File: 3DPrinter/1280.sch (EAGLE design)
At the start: 39 parts, among them IC1 ATMEGA1280-16AU, IC2 7805DT, IC3 CP2102, IC4 X, IC5 Y, IC6 Z, IC7 E0, IC8 E1, J1 22-27-2041-04, J2 22-27-2041-04, J3 22-27-2041-04, J4 22-27-2041-04, J5 22-27-2041-04, Q1 16 MHz, X1 PN61729-S, X2 CON-5.08-03P, X3 CON-5.08-03P, X4 CON-7.62-02P

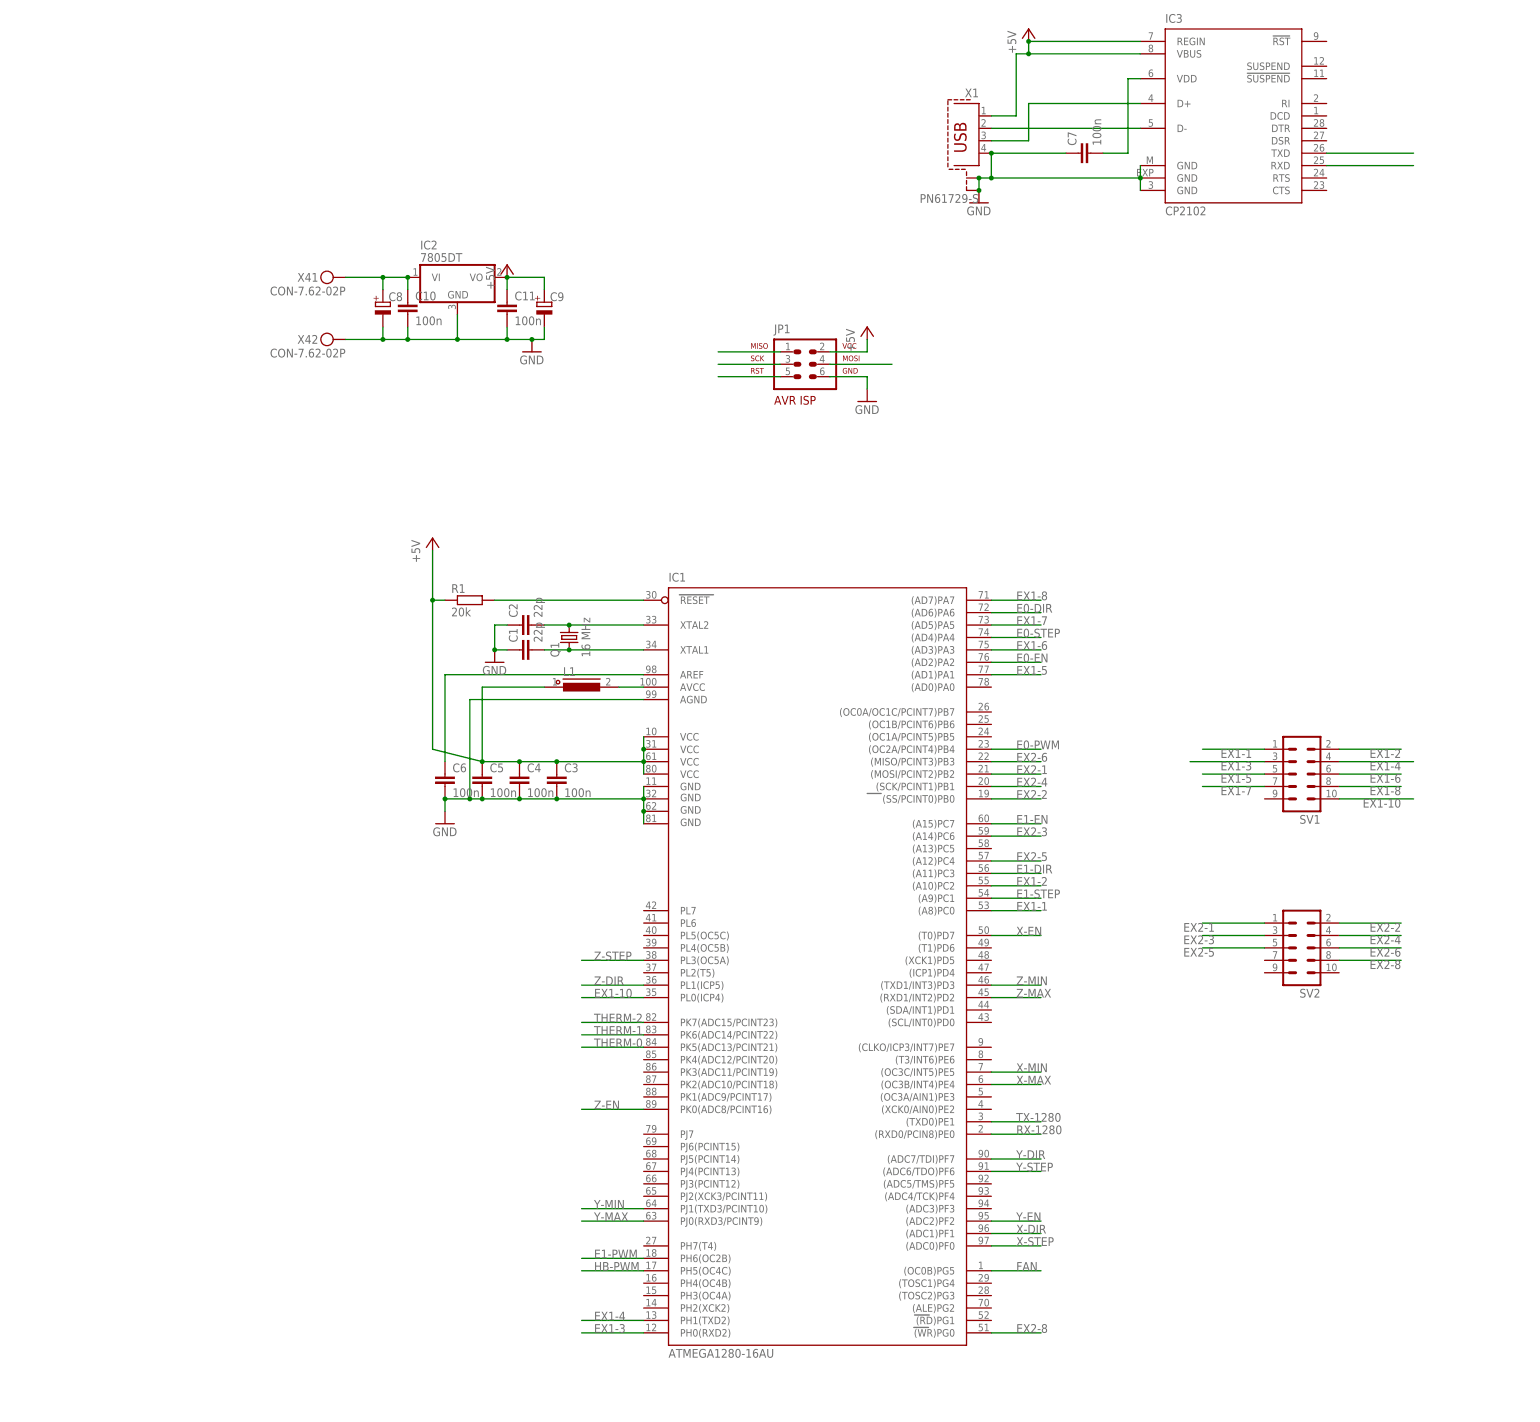
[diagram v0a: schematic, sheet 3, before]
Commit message: полная ардуйня
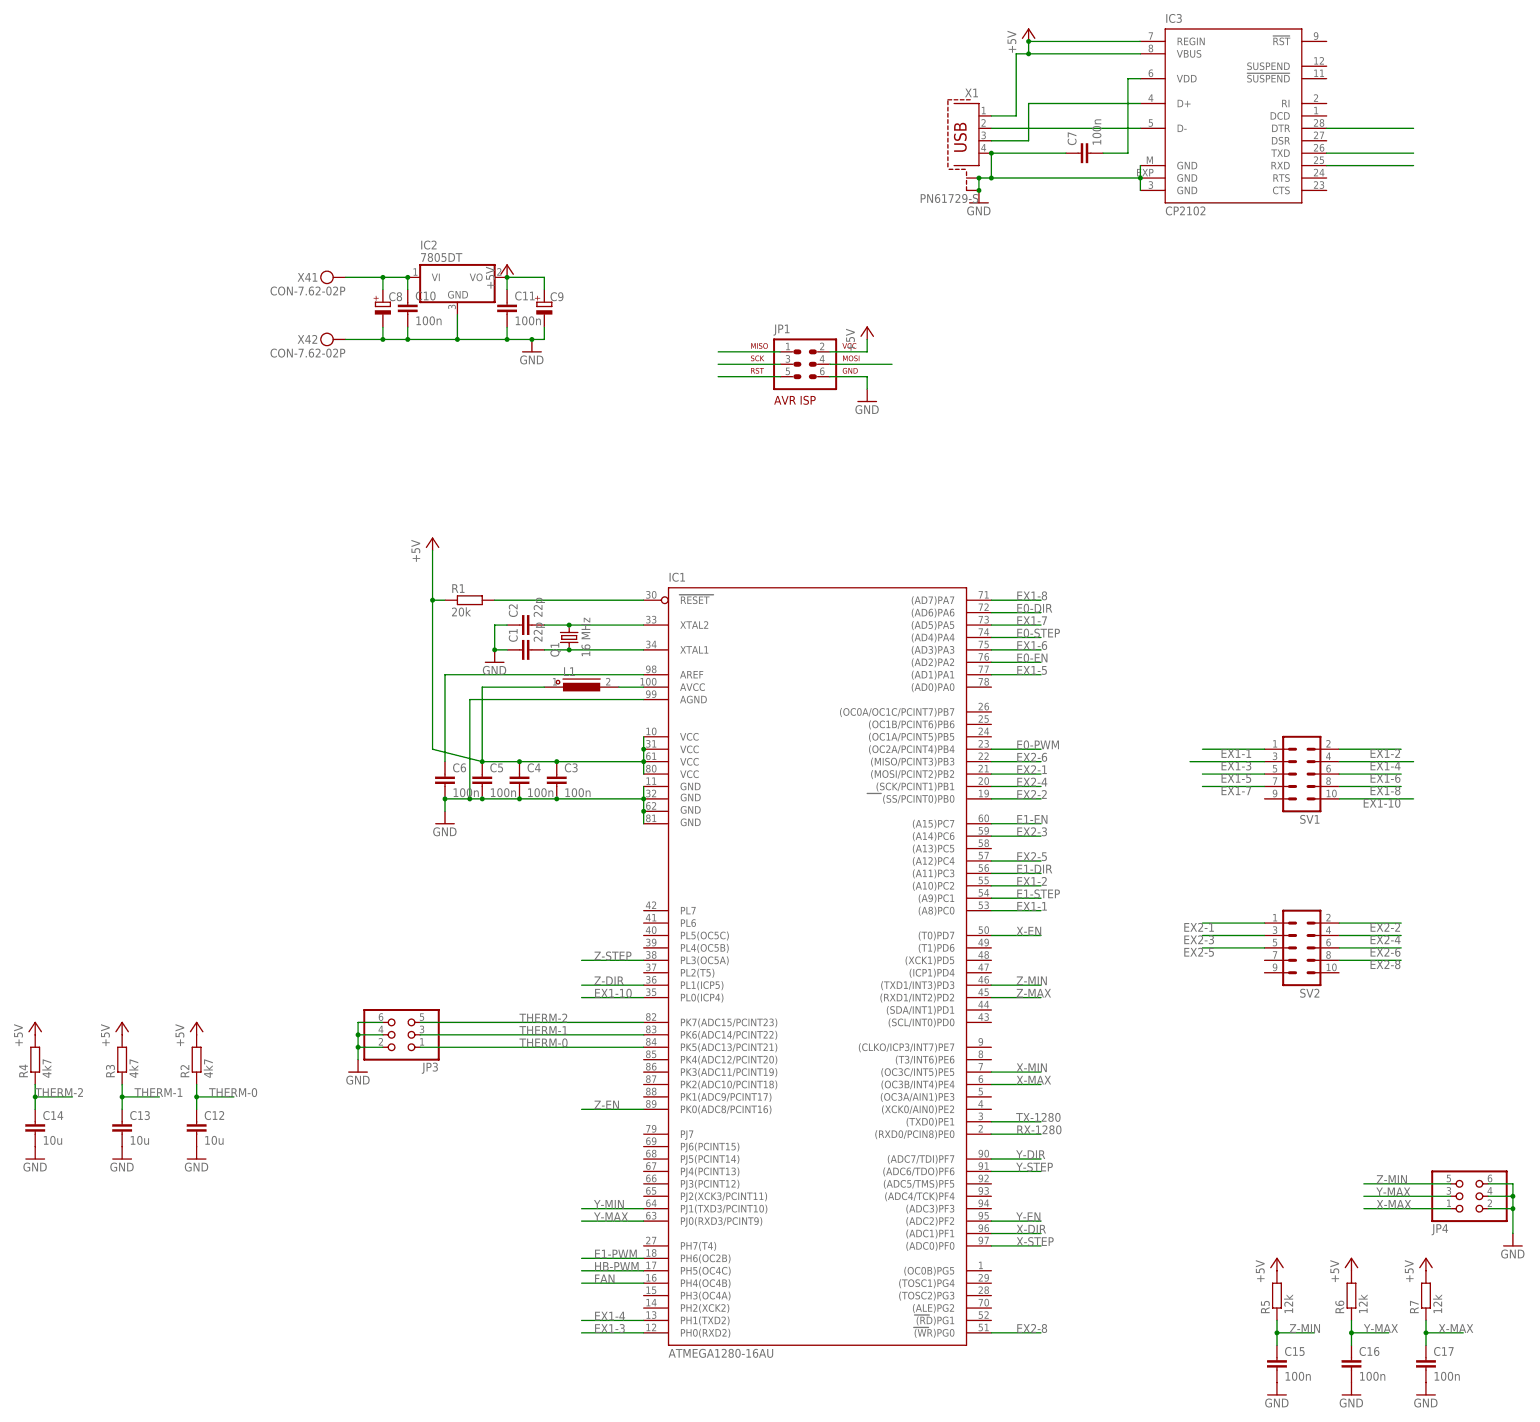
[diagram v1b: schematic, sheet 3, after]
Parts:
- added C12, C13, C14: 10u, Namenlos:CAP_1210
- added C15, C16, C17: 100n, Namenlos:CAP_0805
- added JP3, JP4: (no value), pinhead:PINHD-2X3
- added R2, R3, R4: 4k7, Namenlos:R_0805
- added R5, R6, R7: 12k, Namenlos:R_0805
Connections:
- net !RST: now also IC3.DTR
- net +5V: now also R2.2, R3.2, R4.2, R5.2, R6.2, R7.2
- net FAN: now also IC1.PH4(OC4B); no longer IC1.(OC0B)PG5
- net GND: now also C12.2, C13.2, C14.2, C15.2, C16.2, C17.2, JP3.2, JP3.4, JP3.6, JP4.2, JP4.4, JP4.6
- net THERM-0: now also C12.1, JP3.1, R2.1
- net THERM-1: now also C13.1, JP3.3, R3.1
- net THERM-2: now also C14.1, JP3.5, R4.1
- net X-MAX: now also C17.1, JP4.1, R7.1
- net Y-MAX: now also C16.1, JP4.3, R6.1
- net Z-MIN: now also C15.1, JP4.5, R5.1

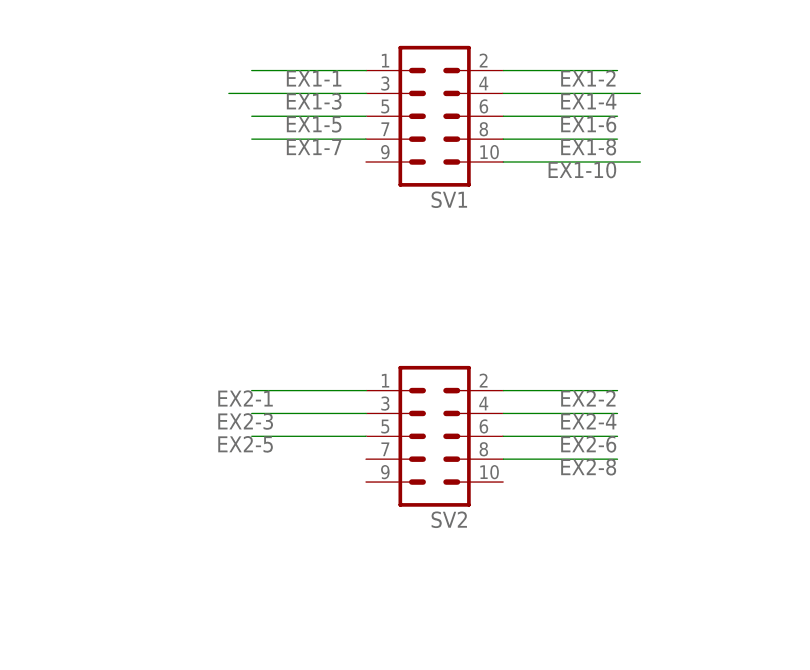
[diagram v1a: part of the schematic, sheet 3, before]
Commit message: _
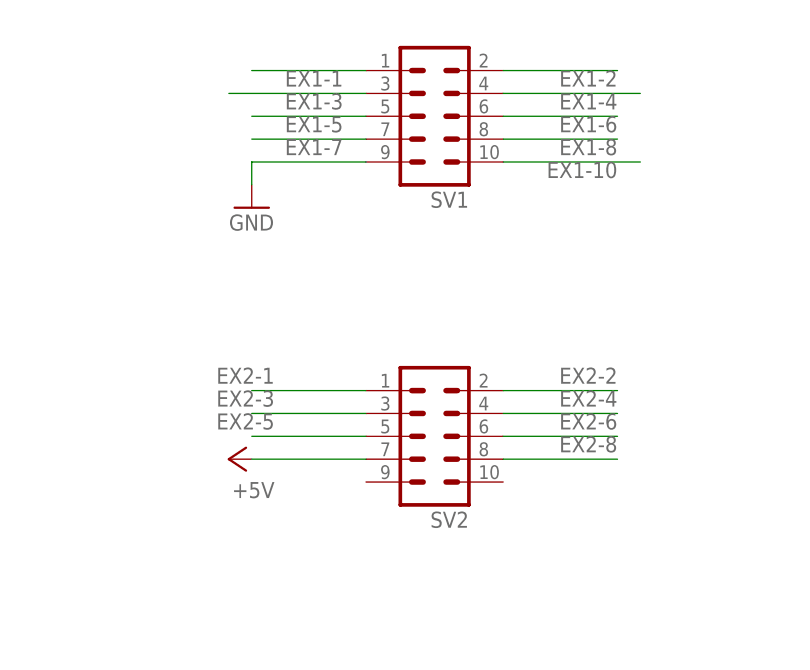
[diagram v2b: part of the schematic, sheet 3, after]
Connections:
- net +5V: now also SV2.7
- net GND: now also SV1.9
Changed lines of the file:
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@@
 <part name="GND26" library="supply1" deviceset="GND" device=""/>
 <part name="GND27" library="supply1" deviceset="GND" device=""/>
+<part name="GND28" library="supply1" deviceset="GND" device=""/>
+<part name="P+16" library="supply1" deviceset="+5V" device=""/>
 </parts>
 <sheets>
@@
 <instance part="GND26" gate="1" x="180.34" y="-48.26"/>
 <instance part="GND27" gate="1" x="198.12" y="-17.78"/>
+<instance part="GND28" gate="1" x="134.62" y="68.58"/>
+<instance part="P+16" gate="1" x="132.08" y="40.64" rot="R90"/>
 </instances>
 <busses>
@@
 <wire x1="134.62" y1="45.72" x2="147.32" y2="45.72" width="0.1524" layer="91"/>
 <pinref part="SV2" gate="G$1" pin="3"/>
-<label x="137.16" y="45.72" size="1.778" layer="95" rot="R180"/>
+<label x="137.16" y="48.26" size="1.778" layer="95" rot="R180"/>
 </segment>
 </net>
@@
 <wire x1="134.62" y1="43.18" x2="147.32" y2="43.18" width="0.1524" layer="91"/>
 <pinref part="SV2" gate="G$1" pin="5"/>
-<label x="137.16" y="43.18" size="1.778" layer="95" rot="R180"/>
+<label x="137.16" y="45.72" size="1.778" layer="95" rot="R180"/>
 </segment>
 </net>
@@
 <wire x1="162.56" y1="40.64" x2="175.26" y2="40.64" width="0.1524" layer="91"/>
 <pinref part="SV2" gate="G$1" pin="8"/>
-<label x="175.26" y="40.64" size="1.778" layer="95" rot="R180"/>
+<label x="175.26" y="43.18" size="1.778" layer="95" rot="R180"/>
 </segment>
 </net>
@@
 <wire x1="134.62" y1="48.26" x2="147.32" y2="48.26" width="0.1524" layer="91"/>
 <pinref part="SV2" gate="G$1" pin="1"/>
-<label x="137.16" y="48.26" size="1.778" layer="95" rot="R180"/>
+<label x="137.16" y="50.8" size="1.778" layer="95" rot="R180"/>
 </segment>
 </net>
@@
 <wire x1="162.56" y1="48.26" x2="175.26" y2="48.26" width="0.1524" layer="91"/>
 <pinref part="SV2" gate="G$1" pin="2"/>
-<label x="175.26" y="48.26" size="1.778" layer="95" rot="R180"/>
+<label x="175.26" y="50.8" size="1.778" layer="95" rot="R180"/>
 </segment>
 </net>
@@
 <wire x1="162.56" y1="45.72" x2="175.26" y2="45.72" width="0.1524" layer="91"/>
 <pinref part="SV2" gate="G$1" pin="4"/>
-<label x="175.26" y="45.72" size="1.778" layer="95" rot="R180"/>
+<label x="175.26" y="48.26" size="1.778" layer="95" rot="R180"/>
 </segment>
 </net>
@@
 <wire x1="162.56" y1="43.18" x2="175.26" y2="43.18" width="0.1524" layer="91"/>
 <pinref part="SV2" gate="G$1" pin="6"/>
-<label x="175.26" y="43.18" size="1.778" layer="95" rot="R180"/>
+<label x="175.26" y="45.72" size="1.778" layer="95" rot="R180"/>
 </segment>
 </net>
@@
 <junction x="198.12" y="-7.62"/>
 </segment>
+<segment>
+<pinref part="SV1" gate="G$1" pin="9"/>
+<wire x1="147.32" y1="73.66" x2="134.62" y2="73.66" width="0.1524" layer="91"/>
+<wire x1="134.62" y1="73.66" x2="134.62" y2="71.12" width="0.1524" layer="91"/>
+<pinref part="GND28" gate="1" pin="GND"/>
+</segment>
 </net>
 <net name="XTAL1" class="0">
@@
 <pinref part="P+15" gate="1" pin="+5V"/>
 </segment>
-</net>
+<segment>
+<pinref part="SV2" gate="G$1" pin="7"/>
+<wire x1="147.32" y1="40.64" x2="134.62" y2="40.64" width="0.1524" layer="91"/>
+<pinref part="P+16" gate="1" pin="+5V"/>
+</segment>
+</net>
